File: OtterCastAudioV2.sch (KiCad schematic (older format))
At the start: 21 parts, among them J1 UART, J2 SD, U1 AllWinner-S3(FBGA-234)

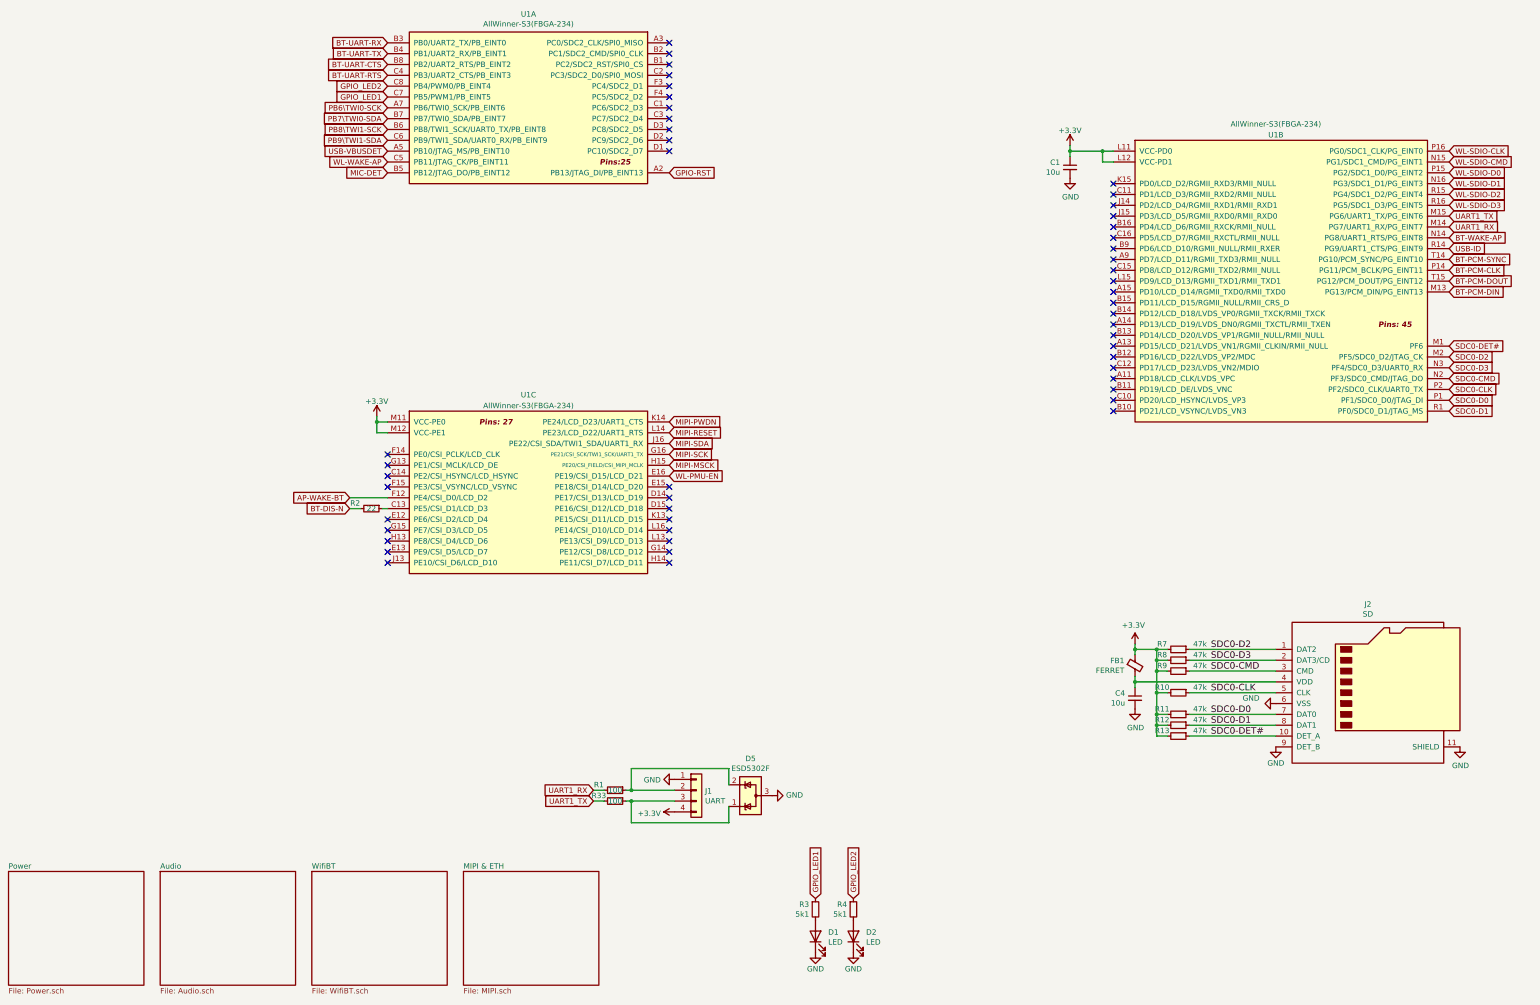
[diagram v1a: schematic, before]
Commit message: beautify kicad project
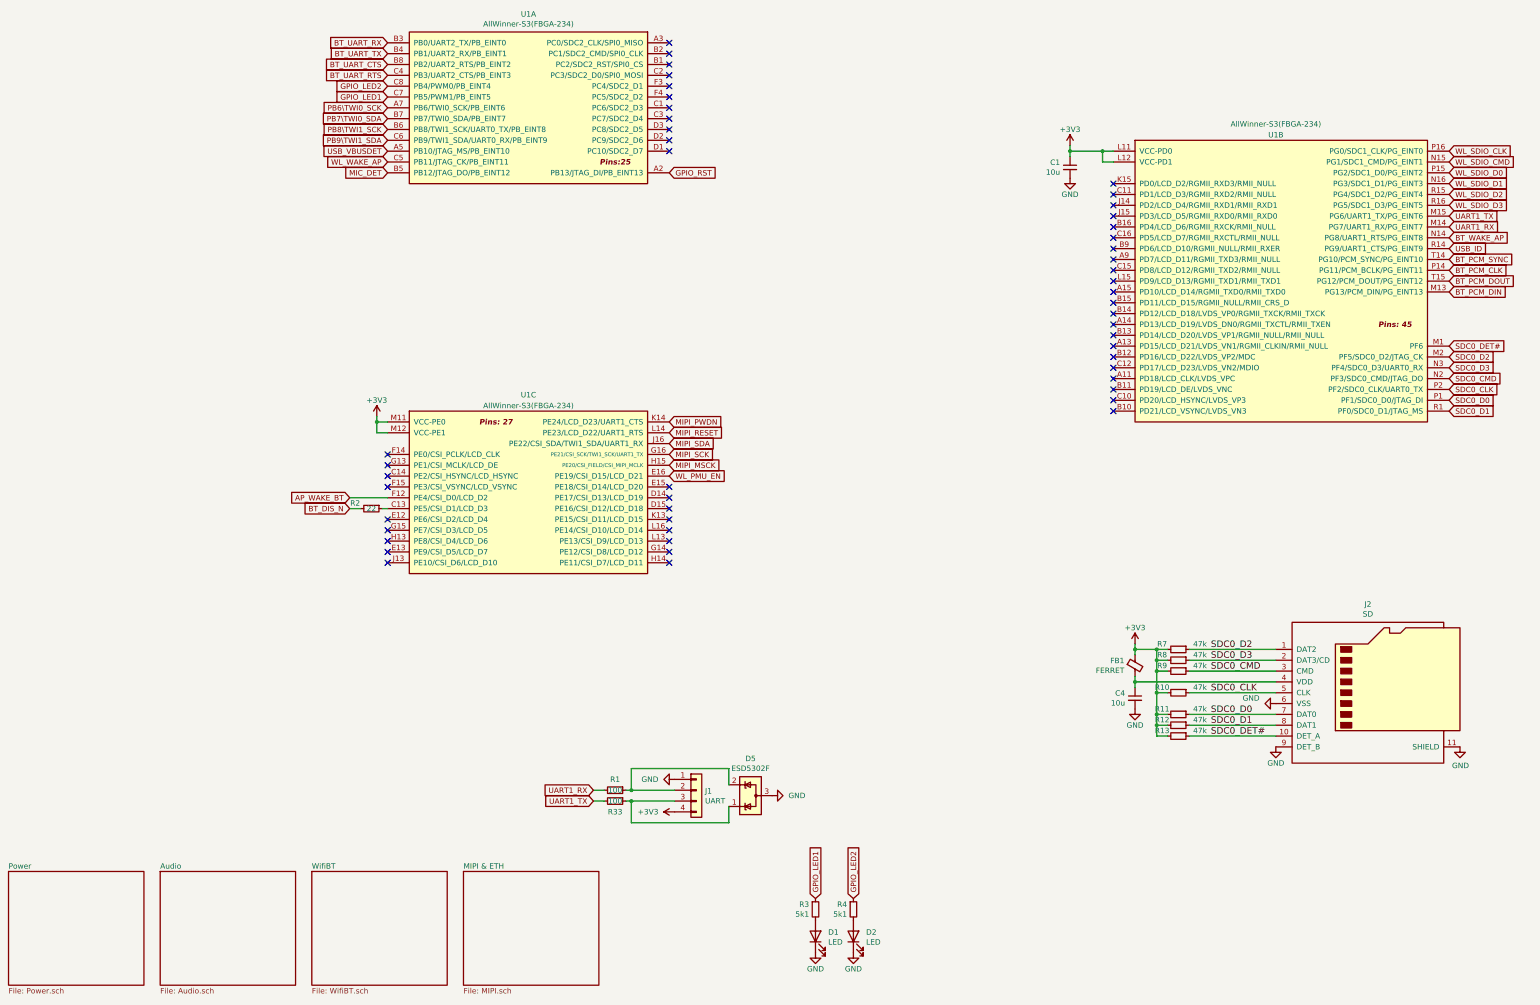
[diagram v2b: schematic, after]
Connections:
- net AP-WAKE-BT renamed AP_WAKE_BT
- net BT-DIS-N renamed BT_DIS_N
- net BT-PCM-CLK renamed BT_PCM_CLK
- net BT-PCM-DIN renamed BT_PCM_DIN
- net BT-PCM-DOUT renamed BT_PCM_DOUT
- net BT-PCM-SYNC renamed BT_PCM_SYNC
- net BT-UART-CTS renamed BT_UART_CTS
- net BT-UART-RTS renamed BT_UART_RTS
- net BT-UART-RX renamed BT_UART_RX
- net BT-UART-TX renamed BT_UART_TX
- net BT-WAKE-AP renamed BT_WAKE_AP
- net GPIO-RST renamed GPIO_RST
- net MIC-DET renamed MIC_DET
- net MIPI-MSCK renamed MIPI_MSCK
- net MIPI-PWDN renamed MIPI_PWDN
- net MIPI-RESET renamed MIPI_RESET
- net MIPI-SCK renamed MIPI_SCK
- net MIPI-SDA renamed MIPI_SDA
- net PB6\TWI0-SCK renamed PB6\TWI0_SCK
- net PB7\TWI0-SDA renamed PB7\TWI0_SDA
- net PB8\TWI1-SCK renamed PB8\TWI1_SCK
- net PB9\TWI1-SDA renamed PB9\TWI1_SDA
- net SDC0-CLK renamed SDC0_CLK
- net SDC0-CMD renamed SDC0_CMD
- net SDC0-D0 renamed SDC0_D0
- net SDC0-D1 renamed SDC0_D1
- net SDC0-D2 renamed SDC0_D2
- net SDC0-D3 renamed SDC0_D3
- net SDC0-DET# renamed SDC0_DET#
- net USB-ID renamed USB_ID
- net USB-VBUSDET renamed USB_VBUSDET
- net WL-PMU-EN renamed WL_PMU_EN
- net WL-SDIO-CLK renamed WL_SDIO_CLK
- net WL-SDIO-CMD renamed WL_SDIO_CMD
- net WL-SDIO-D0 renamed WL_SDIO_D0
- net WL-SDIO-D1 renamed WL_SDIO_D1
- net WL-SDIO-D2 renamed WL_SDIO_D2
- net WL-SDIO-D3 renamed WL_SDIO_D3
- net WL-WAKE-AP renamed WL_WAKE_AP
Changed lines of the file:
@@
 Comment4 ""
 $EndDescr
-$Comp
-L OtterCastAudioV2-rescue:+3.3V-S3-OLinuXino_Rev_A #PWR046
-U 1 1 5D97B54A
-P 10450 3250
-F 0 "#PWR046" H 10450 3100 50  0001 C CNN
-F 1 "+3.3V" H 10450 3390 50  0000 C CNN
-F 2 "" H 10450 3250 60  0000 C CNN
-F 3 "" H 10450 3250 60  0000 C CNN
-	1    10450 3250
-	-1   0    0    -1
-$EndComp
 Wire Wire Line
 	10450 3250 10450 3300
@@
 	10750 3400 10850 3400
 $Comp
-L OtterCastAudioV2-rescue:GND-S3-OLinuXino_Rev_A #PWR047
+L power:GND #PWR047
 U 1 1 57966C0E
 P 8100 10700
@@
 $EndComp
 $Comp
-L OtterCastAudioV2-rescue:GND-S3-OLinuXino_Rev_A #PWR0102
+L power:GND #PWR0102
 U 1 1 6253EB67
 P 12350 8800
@@
 $EndComp
 Text Label 11750 8300 0    60   ~ 0
-SDC0-CLK
+SDC0_CLK
 Text Label 11750 8700 0    60   ~ 0
-SDC0-DET#
+SDC0_DET#
 Text Label 11750 8500 0    60   ~ 0
-SDC0-D0
+SDC0_D0
 Text Label 11750 8600 0    60   ~ 0
-SDC0-D1
+SDC0_D1
 Text Label 11750 7900 0    60   ~ 0
-SDC0-D2
+SDC0_D2
 Text Label 11750 8000 0    60   ~ 0
-SDC0-D3
+SDC0_D3
 Text Label 11750 8100 0    60   ~ 0
-SDC0-CMD
+SDC0_CMD
 $Comp
 L Device:R_Small R7
@@
 P 11050 8450
 F 0 "#PWR0104" H 11050 8200 50  0001 C CNN
-F 1 "GND" H 11055 8277 50  0000 C CNN
+F 1 "GND" H 11050 8300 50  0000 C CNN
 F 2 "" H 11050 8450 60  0000 C CNN
 F 3 "" H 11050 8450 60  0000 C CNN
@@
 Wire Wire Line
 	11050 8200 12350 8200
-$Comp
-L OtterCastAudioV2-rescue:+3.3V-S3-OLinuXino_Rev_A #PWR0105
-U 1 1 62FAA3E6
-P 11050 7850
-F 0 "#PWR0105" H 11050 7700 50  0001 C CNN
-F 1 "+3.3V" H 11065 8023 50  0000 C CNN
-F 2 "" H 11050 7850 60  0000 C CNN
-F 3 "" H 11050 7850 60  0000 C CNN
-	1    11050 7850
-	-1   0    0    -1
-$EndComp
 Wire Wire Line
 	11050 8150 11050 8200
@@
 P 10450 3550
 F 0 "#PWR0106" H 10450 3300 50  0001 C CNN
-F 1 "GND" H 10455 3377 50  0000 C CNN
+F 1 "GND" H 10450 3400 50  0000 C CNN
 F 2 "" H 10450 3550 60  0000 C CNN
 F 3 "" H 10450 3550 60  0000 C CNN
@@
 NoConn ~ 10850 5700
 Text GLabel 13950 5100 2    50   Input ~ 0
-SDC0-DET#
+SDC0_DET#
 Text GLabel 13950 5200 2    50   Input ~ 0
-SDC0-D2
+SDC0_D2
 Text GLabel 13950 5300 2    50   Input ~ 0
-SDC0-D3
+SDC0_D3
 Text GLabel 13950 5400 2    50   Input ~ 0
-SDC0-CMD
+SDC0_CMD
 Text GLabel 13950 5600 2    50   Input ~ 0
-SDC0-D0
+SDC0_D0
 Text GLabel 13950 5700 2    50   Input ~ 0
-SDC0-D1
+SDC0_D1
 Text GLabel 13950 5500 2    50   Input ~ 0
-SDC0-CLK
+SDC0_CLK
 Text GLabel 13950 3300 2    50   Input ~ 0
-WL-SDIO-CLK
+WL_SDIO_CLK
 Text GLabel 13950 3400 2    50   Input ~ 0
-WL-SDIO-CMD
+WL_SDIO_CMD
 Text GLabel 13950 3500 2    50   Input ~ 0
-WL-SDIO-D0
+WL_SDIO_D0
 Text GLabel 13950 3600 2    50   Input ~ 0
-WL-SDIO-D1
+WL_SDIO_D1
 Text GLabel 13950 3700 2    50   Input ~ 0
-WL-SDIO-D2
+WL_SDIO_D2
 Text GLabel 13950 3800 2    50   Input ~ 0
-WL-SDIO-D3
+WL_SDIO_D3
 Text GLabel 13950 3900 2    50   Input ~ 0
 UART1_TX
@@
 UART1_RX
 Text GLabel 13950 4100 2    50   Input ~ 0
-BT-WAKE-AP
+BT_WAKE_AP
 Text GLabel 13950 4300 2    50   Input ~ 0
-BT-PCM-SYNC
+BT_PCM_SYNC
 Text GLabel 13950 4400 2    50   Input ~ 0
-BT-PCM-CLK
+BT_PCM_CLK
 Text GLabel 13950 4600 2    50   Input ~ 0
-BT-PCM-DIN
+BT_PCM_DIN
 Text GLabel 13950 4500 2    50   Input ~ 0
-BT-PCM-DOUT
+BT_PCM_DOUT
 $Comp
 L Connector_Generic:Conn_01x04 J1
@@
 P 6800 9100
 F 0 "#PWR0107" H 6800 8850 50  0001 C CNN
-F 1 "GND" V 6805 8972 50  0000 R CNN
+F 1 "GND" V 6800 8950 50  0000 R CNN
 F 2 "" H 6800 9100 60  0000 C CNN
 F 3 "" H 6800 9100 60  0000 C CNN
@@
 Text GLabel 6050 9200 0    50   Input ~ 0
 UART1_RX
-$Comp
-L OtterCastAudioV2-rescue:+3.3V-S3-OLinuXino_Rev_A #PWR0108
-U 1 1 63623CC5
-P 6800 9400
-F 0 "#PWR0108" H 6800 9250 50  0001 C CNN
-F 1 "+3.3V" V 6815 9528 50  0000 L CNN
-F 2 "" H 6800 9400 60  0000 C CNN
-F 3 "" H 6800 9400 60  0000 C CNN
-	1    6800 9400
-	0    -1   1    0
-$EndComp
 Text GLabel 4150 2800 0    50   Input ~ 0
 GPIO_LED1
@@
 $EndComp
 Text GLabel 3800 6500 0    50   Input ~ 0
-AP-WAKE-BT
+AP_WAKE_BT
 Text GLabel 3800 6600 0    50   Input ~ 0
-BT-DIS-N
+BT_DIS_N
 $Comp
 L Device:R_Small R2
@@
 NoConn ~ 4150 7100
 Text GLabel 6750 6300 2    50   Input ~ 0
-WL-PMU-EN
+WL_PMU_EN
 Text GLabel 6750 6000 2    50   Input ~ 0
-MIPI-SDA
+MIPI_SDA
 Text GLabel 6750 6100 2    50   Input ~ 0
-MIPI-SCK
+MIPI_SCK
 Text GLabel 6750 5900 2    50   Input ~ 0
-MIPI-RESET
+MIPI_RESET
 Text GLabel 6750 5800 2    50   Input ~ 0
-MIPI-PWDN
-$Comp
-L OtterCastAudioV2-rescue:+3.3V-S3-OLinuXino_Rev_A #PWR0109
-U 1 1 63B28C18
-P 4050 5750
-F 0 "#PWR0109" H 4050 5600 50  0001 C CNN
-F 1 "+3.3V" H 4050 5890 50  0000 C CNN
-F 2 "" H 4050 5750 60  0000 C CNN
-F 3 "" H 4050 5750 60  0000 C CNN
-	1    4050 5750
-	-1   0    0    -1
-$EndComp
+MIPI_PWDN
 Wire Wire Line
 	4050 5750 4050 5800
@@
 GPIO_LED2
 $Comp
-L OtterCastAudioV2-rescue:GND-S3-OLinuXino_Rev_A #PWR0111
+L power:GND #PWR0111
 U 1 1 67BFC606
 P 8450 10700
@@
 $EndComp
 Text GLabel 4150 2300 0    50   Input ~ 0
-BT-UART-RX
+BT_UART_RX
 Text GLabel 4150 2400 0    50   Input ~ 0
-BT-UART-TX
+BT_UART_TX
 Text GLabel 4150 2500 0    50   Input ~ 0
-BT-UART-CTS
+BT_UART_CTS
 Text GLabel 4150 2900 0    50   Input ~ 0
-PB6\TWI0-SCK
+PB6\TWI0_SCK
 Text GLabel 4150 3000 0    50   Input ~ 0
-PB7\TWI0-SDA
+PB7\TWI0_SDA
 Text GLabel 4150 3100 0    50   Input ~ 0
-PB8\TWI1-SCK
+PB8\TWI1_SCK
 Text GLabel 4150 3200 0    50   Input ~ 0
-PB9\TWI1-SDA
+PB9\TWI1_SDA
 Text GLabel 4150 3300 0    50   Input ~ 0
-USB-VBUSDET
+USB_VBUSDET
 Text GLabel 4150 3400 0    50   Input ~ 0
-WL-WAKE-AP
+WL_WAKE_AP
 Text GLabel 4150 3500 0    50   Input ~ 0
-MIC-DET
+MIC_DET
 Text GLabel 13950 4200 2    50   Input ~ 0
-USB-ID
+USB_ID
 Text GLabel 6750 6200 2    50   Input ~ 0
-MIPI-MSCK
+MIPI_MSCK
 $Comp
 L otter:AllWinner-S3(FBGA-234) U1
@@
 $EndComp
 Text GLabel 4150 2600 0    50   Input ~ 0
-BT-UART-RTS
+BT_UART_RTS
 $Comp
 L Device:R_Small R1
 U 1 1 5FE69B36
 P 6250 9200
-F 0 "R1" V 6200 9050 50  0000 C CNN
+F 0 "R1" V 6150 9200 50  0000 C CNN
 F 1 "100" V 6250 9200 50  0000 C CNN
 F 2 "otter:R_0402" H 6250 9200 50  0001 C CNN
@@
 U 1 1 5FE69B3C
 P 6250 9300
-F 0 "R33" V 6200 9150 50  0000 C CNN
+F 0 "R33" V 6350 9300 50  0000 C CNN
 F 1 "100" V 6250 9300 50  0000 C CNN
 F 2 "otter:R_0402" H 6250 9300 50  0001 C CNN
@@
 	6400 9200 6800 9200
 Text GLabel 6750 3500 2    50   Input ~ 0
-GPIO-RST
+GPIO_RST
 $Comp
 L otter:GND #PWR0110
@@
 P 7700 9250
 F 0 "#PWR0110" H 7700 9000 50  0001 C CNN
-F 1 "GND" V 7705 9122 50  0000 R CNN
+F 1 "GND" V 7700 9100 50  0000 R CNN
 F 2 "" H 7700 9250 60  0000 C CNN
 F 3 "" H 7700 9250 60  0000 C CNN
@@
 	0    -1   -1   0
 $EndComp
+$Comp
+L power:+3V3 #PWR?
+U 1 1 604123F5
+P 4050 5750
+AR Path="/604A1CEE/604123F5" Ref="#PWR?"  Part="1"
+AR Path="/604123F5" Ref="#PWR?"  Part="1"
+F 0 "#PWR?" H 4050 5600 50  0001 C CNN
+F 1 "+3V3" H 4050 5900 50  0000 C CNN
+F 2 "" H 4050 5750 50  0001 C CNN
+F 3 "" H 4050 5750 50  0001 C CNN
+	1    4050 5750
+	1    0    0    -1
+$EndComp
+$Comp
+L power:+3V3 #PWR?
+U 1 1 604143DF
+P 10450 3250
+AR Path="/604A1CEE/604143DF" Ref="#PWR?"  Part="1"
+AR Path="/604143DF" Ref="#PWR?"  Part="1"
+F 0 "#PWR?" H 10450 3100 50  0001 C CNN
+F 1 "+3V3" H 10450 3400 50  0000 C CNN
+F 2 "" H 10450 3250 50  0001 C CNN
+F 3 "" H 10450 3250 50  0001 C CNN
+	1    10450 3250
+	1    0    0    -1
+$EndComp
+$Comp
+L power:+3V3 #PWR?
+U 1 1 604162DF
+P 11050 7850
+AR Path="/604A1CEE/604162DF" Ref="#PWR?"  Part="1"
+AR Path="/604162DF" Ref="#PWR?"  Part="1"
+F 0 "#PWR?" H 11050 7700 50  0001 C CNN
+F 1 "+3V3" H 11050 8000 50  0000 C CNN
+F 2 "" H 11050 7850 50  0001 C CNN
+F 3 "" H 11050 7850 50  0001 C CNN
+	1    11050 7850
+	1    0    0    -1
+$EndComp
+$Comp
+L power:+3V3 #PWR?
+U 1 1 60453D8B
+P 6800 9400
+AR Path="/604A1CEE/60453D8B" Ref="#PWR?"  Part="1"
+AR Path="/60453D8B" Ref="#PWR?"  Part="1"
+F 0 "#PWR?" H 6800 9250 50  0001 C CNN
+F 1 "+3V3" V 6800 9550 50  0000 L CNN
+F 2 "" H 6800 9400 50  0001 C CNN
+F 3 "" H 6800 9400 50  0001 C CNN
+	1    6800 9400
+	0    -1   -1   0
+$EndComp
